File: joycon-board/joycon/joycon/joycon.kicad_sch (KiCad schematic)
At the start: 11 parts, among them J1 Conn_01x05_Male, J10 Conn_01x01_Female, J11 Conn_01x01_Female, J2 Conn_01x05_Female, J3 Conn_01x01_Female, J4 Conn_01x01_Female, J5 Conn_01x01_Female, J6 Conn_01x01_Female, J7 Conn_01x02_Female, J8 Conn_01x01_Female, J9 Conn_01x01_Female

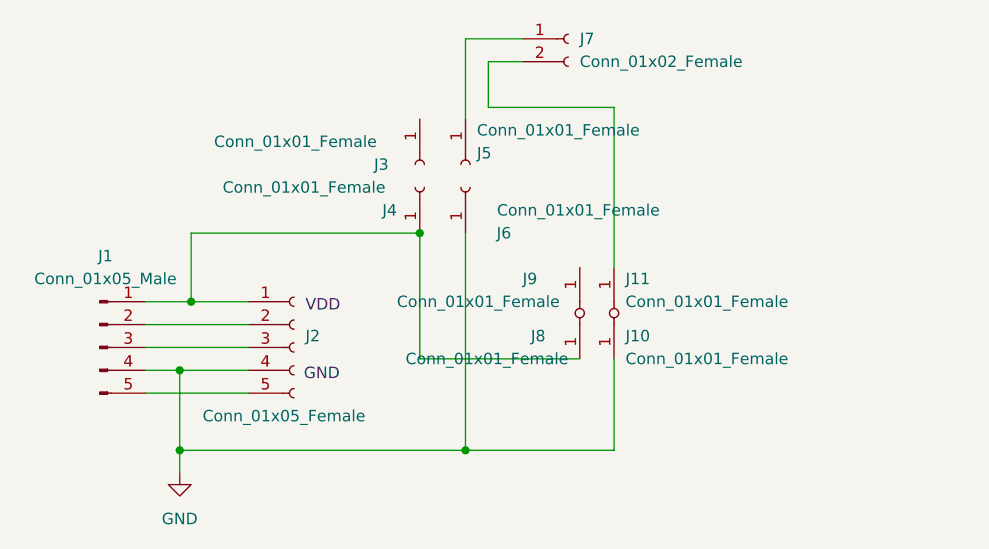
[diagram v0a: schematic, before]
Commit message: joystick-PCB
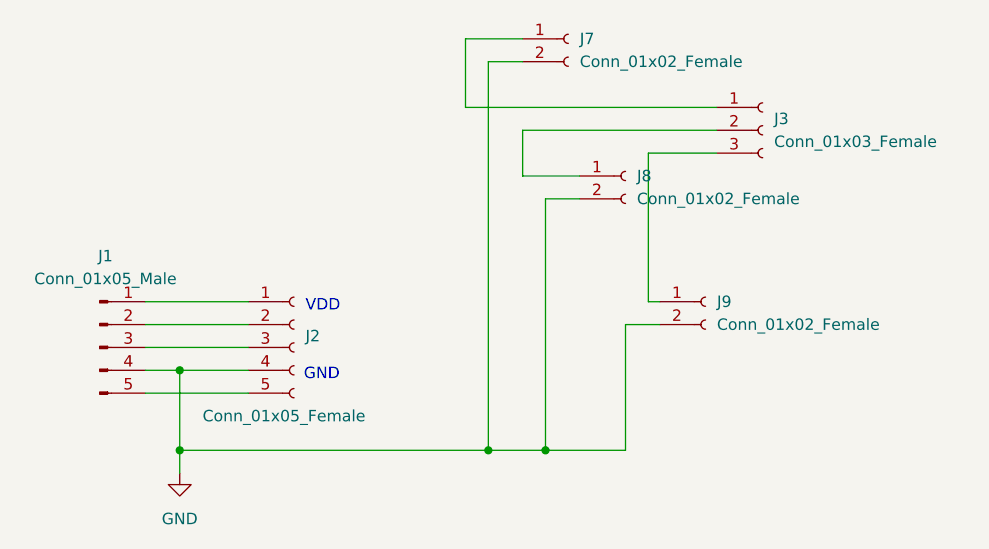
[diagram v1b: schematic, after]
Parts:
- removed J10, J11, J3, J4, J5, J6, J8, J9: Conn_01x01_Female, Connector_PinSocket_1.27mm:PinSocket_1x01_P1.27mm_Vertical, symbol Connector:Conn_01x01_Female
- added J3: Conn_01x03_Female, Connector_PinSocket_2.54mm:PinSocket_1x03_P2.54mm_Vertical, symbol Connector:Conn_01x03_Female
- added J8, J9: Conn_01x02_Female, Connector_PinSocket_2.54mm:PinSocket_1x02_P2.54mm_Vertical, symbol Connector:Conn_01x02_Female
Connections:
- net GND: now also J7.2 (Pin_2), J8.2 (Pin_2), J9.2 (Pin_2)
- net at J7.1 (Pin_1): now also J3.1 (Pin_1)
- new net: J3.2 (Pin_2), J8.1 (Pin_1)
- new net: J3.3 (Pin_3), J9.1 (Pin_1)
